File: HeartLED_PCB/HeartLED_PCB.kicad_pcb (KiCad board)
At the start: 2 copper layers, 58.8 x 52.2 mm, 37 parts, among them U1 ICM7555IBAZ-T, U2 CD4017BM96, U3 TPS61222DCKR, U4 HX SS12F44G4

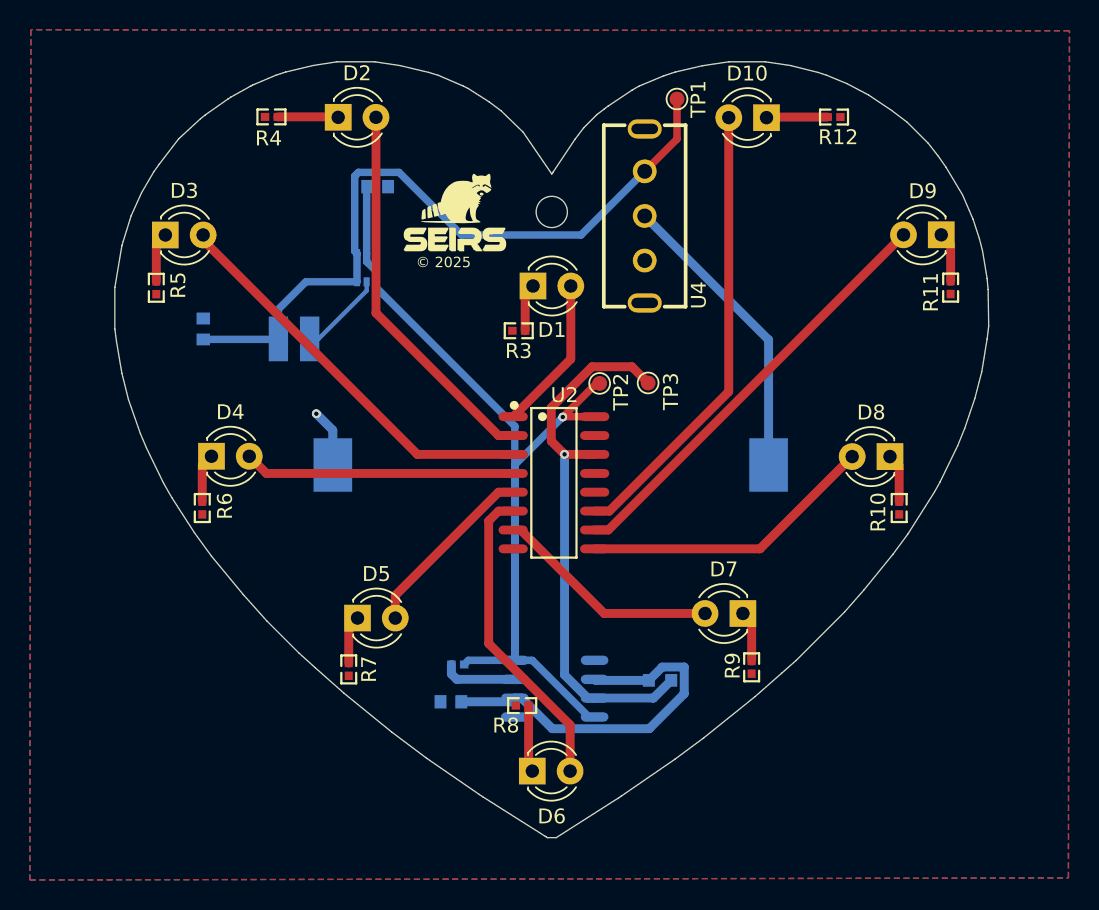
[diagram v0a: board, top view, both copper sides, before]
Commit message: Routing done
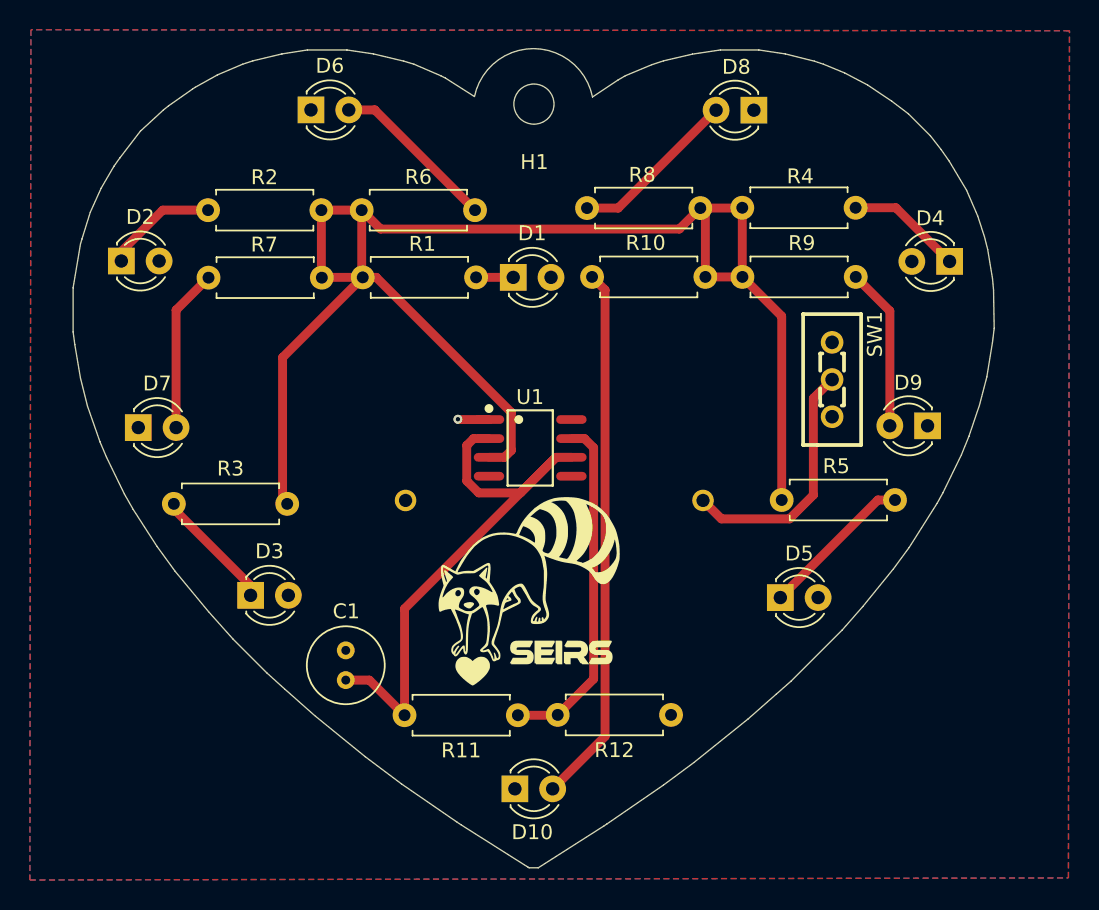
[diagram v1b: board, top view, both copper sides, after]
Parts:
- removed BT1: Battery_Cell, Battery:BatteryHolder_Keystone_1060_1x2032
- removed C2, C3: 10uF, FOOTPRINTS:CL10A106MQ8NNNC
- removed the G*** at (123.5, 81.7)
- removed L1: 4.7uH, FOOTPRINTS:LQH3NPN4R7MMEL
- removed TP1, TP2, TP3: TestPoint, TestPoint:TestPoint_Pad_D1.0mm
- removed U3: TPS61222DCKR, FOOTPRINTS:TPS61222DCKR
- removed U4: HX SS12F44G4, FOOTPRINTS:HX SS12F44G4
- added G***: LOGO, FOOTPRINTS:raccoon, F.Cu at (128.5, 108.1)
- added SW1: SS12D00G3, FOOTPRINTS:SS12D00G3, F.Cu at (148.8, 93.9)
- C1: value 4.7uF -> 47uF; footprint FOOTPRINTS:CL10A475KP8NNNC -> Capacitor_THT:C_Radial_D5.0mm_H7.0mm_P2.00mm; moved to F.Cu
- H1: footprint MountingHole:MountingHole_2.1mm -> MountingHole:MountingHole_2.7mm
- R1: value 100k -> 1k; footprint FOOTPRINTS:0603WAJ0104T5E -> Resistor_THT:R_Axial_DIN0207_L6.3mm_D2.5mm_P7.62mm_Horizontal; moved to F.Cu
- R10, R3, R4, R5, R6, R7, R8, R9: value 3.3k -> 1k; footprint FOOTPRINTS:0402WGJ0332TCE -> Resistor_THT:R_Axial_DIN0207_L6.3mm_D2.5mm_P7.62mm_Horizontal
- R11: value 3.3k -> 10K; footprint FOOTPRINTS:0402WGJ0332TCE -> Resistor_THT:R_Axial_DIN0207_L6.3mm_D2.5mm_P7.62mm_Horizontal
- R12: value 3.3k -> 1OK; footprint FOOTPRINTS:0402WGJ0332TCE -> Resistor_THT:R_Axial_DIN0207_L6.3mm_D2.5mm_P7.62mm_Horizontal
- R2: value 10k -> 1k; footprint FOOTPRINTS:0402WGJ0103TCE -> Resistor_THT:R_Axial_DIN0207_L6.3mm_D2.5mm_P7.62mm_Horizontal; moved to F.Cu
- U1: value ICM7555IBAZ-T -> NE555DR; footprint FOOTPRINTS:ICM7555IBAZ-T -> FOOTPRINTS:NE555DR; moved to F.Cu
- U2: value CD4017BM96 -> 1066; footprint FOOTPRINTS:CD4017BM96 -> FOOTPRINTS:1066; moved to B.Cu
- moved R5 51.7 mm to (153.1, 102.0), turned to 180 degrees
- moved D4 51.3 mm to (156.8, 85.9), turned to 180 degrees
- moved D10 48.2 mm to (127.5, 121.4), turned to 0 degrees
- moved D6 46.9 mm to (113.8, 75.7)
- moved D7 42.5 mm to (102.2, 97.1), turned to 0 degrees
- moved R12 41.7 mm to (138.0, 116.4)
- moved R11 40.9 mm to (127.7, 116.4), turned to 180 degrees
- moved R4 39.8 mm to (150.4, 82.3)
- moved R8 35.5 mm to (140.0, 82.3)
- moved R2 34.9 mm to (106.9, 82.5)
- moved R1 29.8 mm to (124.9, 87.0)
- moved G*** 28.7 mm to (130.6, 112.3)
- moved D5 28.5 mm to (145.4, 108.5)
- moved R7 26.4 mm to (114.5, 87.0), turned to 180 degrees
- moved R9 26.3 mm to (142.8, 87.0), turned to 0 degrees
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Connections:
- C1 pad 1: Net-(U1-THRESHOLD) -> Net-(U1-THRES)
- D1 pad 2: Net-(D1-A) -> VCC
- D10 pad 1: Net-(D10-K) -> GND
- D2 pad 2: Net-(D2-A) -> VCC
- D3 pad 2: Net-(D3-A) -> VCC
- D4 pad 2: Net-(D4-A) -> VCC
- D5 pad 2: Net-(D5-A) -> VCC
- D6 pad 1: Net-(D6-K) -> GND
- D7 pad 1: Net-(D7-K) -> GND
- D8 pad 1: Net-(D8-K) -> GND
- D9 pad 1: Net-(D9-K) -> GND
- R1 pad 1: ASTABLE_OUTPUT -> Net-(D1-K)
- R1 pad 2: Net-(U1-THRESHOLD) -> Net-(U1-OUT)
- R10 pad 1: GND -> Net-(U1-OUT)
- R10 pad 2: Net-(D8-K) -> Net-(D10-A)
- R11 pad 1: GND -> Net-(U1-DISCH)
- R11 pad 2: Net-(D9-K) -> Net-(U1-THRES)
- R12 pad 1: GND -> VCC
- R12 pad 2: Net-(D10-K) -> Net-(U1-DISCH)
- R2 pad 1: Net-(U1-DISCHARGE) -> Net-(D2-K)
- R2 pad 2: +5V -> Net-(U1-OUT)
- R3 pad 1: Net-(D1-K) -> Net-(D3-K)
- R3 pad 2: GND -> Net-(U1-OUT)
- R4 pad 1: Net-(D2-K) -> Net-(D4-K)
- R4 pad 2: GND -> Net-(U1-OUT)
- R5 pad 1: Net-(D3-K) -> Net-(D5-K)
- R5 pad 2: GND -> Net-(U1-OUT)
- R6 pad 1: Net-(D4-K) -> Net-(U1-OUT)
- R6 pad 2: GND -> Net-(D6-A)
- R7 pad 1: GND -> Net-(U1-OUT)
- R7 pad 2: Net-(D5-K) -> Net-(D7-A)
- R8 pad 1: Net-(D6-K) -> Net-(U1-OUT)
- R8 pad 2: GND -> Net-(D8-A)
- R9 pad 1: Net-(D7-K) -> Net-(U1-OUT)
- R9 pad 2: GND -> Net-(D9-A)
- U1 pad 2: Net-(U1-THRESHOLD) -> Net-(U1-THRES)
- U1 pad 3: ASTABLE_OUTPUT -> Net-(U1-OUT)
- U1 pad 4: +5V -> VCC
- U1 pad 5: GND -> unconnected-(U1-CONT-Pad5)
- U1 pad 6: Net-(U1-THRESHOLD) -> Net-(U1-THRES)
- U1 pad 7: Net-(U1-DISCHARGE) -> Net-(U1-DISCH)
- U1 pad 8: +5V -> VCC
- U2 pad 1: Net-(D1-A) -> GND
- U2 pad 2: Net-(D2-A) -> Net-(SW1-Pad2)
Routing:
- net Net-(U1-OUT): track 0.00 -> 104.6 mm
- net +5V: track 69.5 -> 0.00 mm, vias 1 -> 0
- net +3V: track 49.1 -> 0.00 mm
- net Net-(U1-THRES): track 0.00 -> 38.9 mm
- net ASTABLE_OUTPUT: track 36.8 -> 0.00 mm, vias 1 -> 0
- net Net-(D3-A): track 27.3 -> 0.00 mm
- net Net-(D2-A): track 25.8 -> 0.00 mm
- net Net-(U1-THRESHOLD): track 25.1 -> 0.00 mm
- net Net-(U1-DISCH): track 0.00 -> 23.4 mm
- net Net-(BT1-+): track 20.2 -> 0.00 mm
- net Net-(D4-A): track 18.2 -> 0.00 mm
- net Net-(D9-A): track 29.0 -> 11.0 mm
- net Net-(SW1-Pad2): track 0.00 -> 16.9 mm
- net Net-(D5-A): track 12.3 -> 0.00 mm
- net Net-(D1-A): track 10.4 -> 0.00 mm
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- added copper zone on F.Cu, net VCC
- removed copper zone on F.Cu, net GND
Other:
- board size 58.8 x 52.2 mm -> 61.9 x 55.1 mm
- board text removed: "Happy Valentine's Day ( ˘ ³˘)♥"
- board text removed: "github.com/ fectec/ HeartLED"
- board text removed: "v1.0.0"
- board text removed: "© 2025"
